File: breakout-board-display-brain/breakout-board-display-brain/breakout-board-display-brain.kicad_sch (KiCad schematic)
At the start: 7 parts, among them J1 Conn_01x19_Socket, J2 Conn_01x19_Socket, J3 Conn_01x02_Socket, J4 Conn_01x04_Socket, J5 Conn_01x04_Socket, SW1 RotaryEncoder_Switch, U1 ESP32-WROOM-32

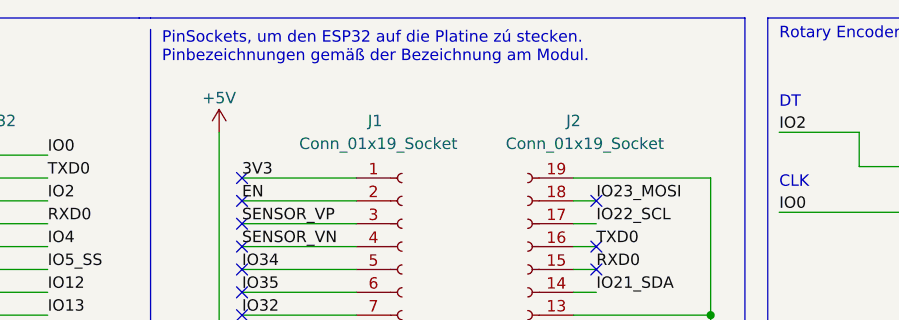
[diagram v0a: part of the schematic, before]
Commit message: ...
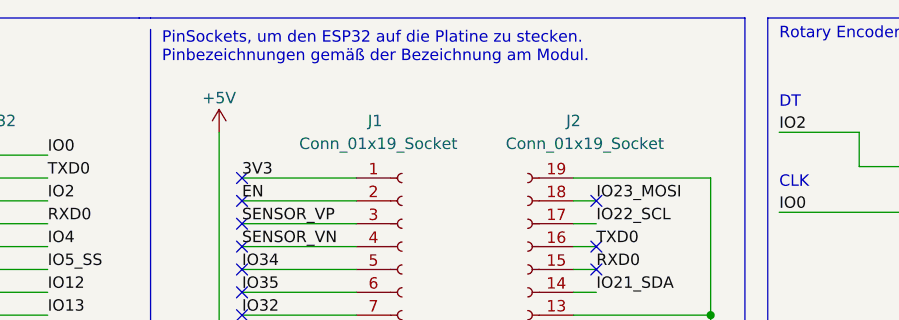
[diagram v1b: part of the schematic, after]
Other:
- note added: "PinSockets, um den ESP32 auf die Platine zu stecken. Pinbezeichnungen gemäß der Bezeichnung am Modul."
- note removed: "PinSockets, um den ESP32 auf die Platine zú stecken. Pinbezeichnungen gemäß der Bezeichnung am Modul."
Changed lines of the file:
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@@
     (effects (font (size 1.27 1.27)) (justify left bottom))
   )
-  (text "PinSockets, um den ESP32 auf die Platine zú stecken.\nPinbezeichnungen gemäß der Bezeichnung am Modul."
+  (text "PinSockets, um den ESP32 auf die Platine zu stecken.\nPinbezeichnungen gemäß der Bezeichnung am Modul."
     (at 101.6 19.05 0)
     (effects (font (size 1.27 1.27)) (justify left bottom))
